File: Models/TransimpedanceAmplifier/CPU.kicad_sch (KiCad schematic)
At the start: 0 parts

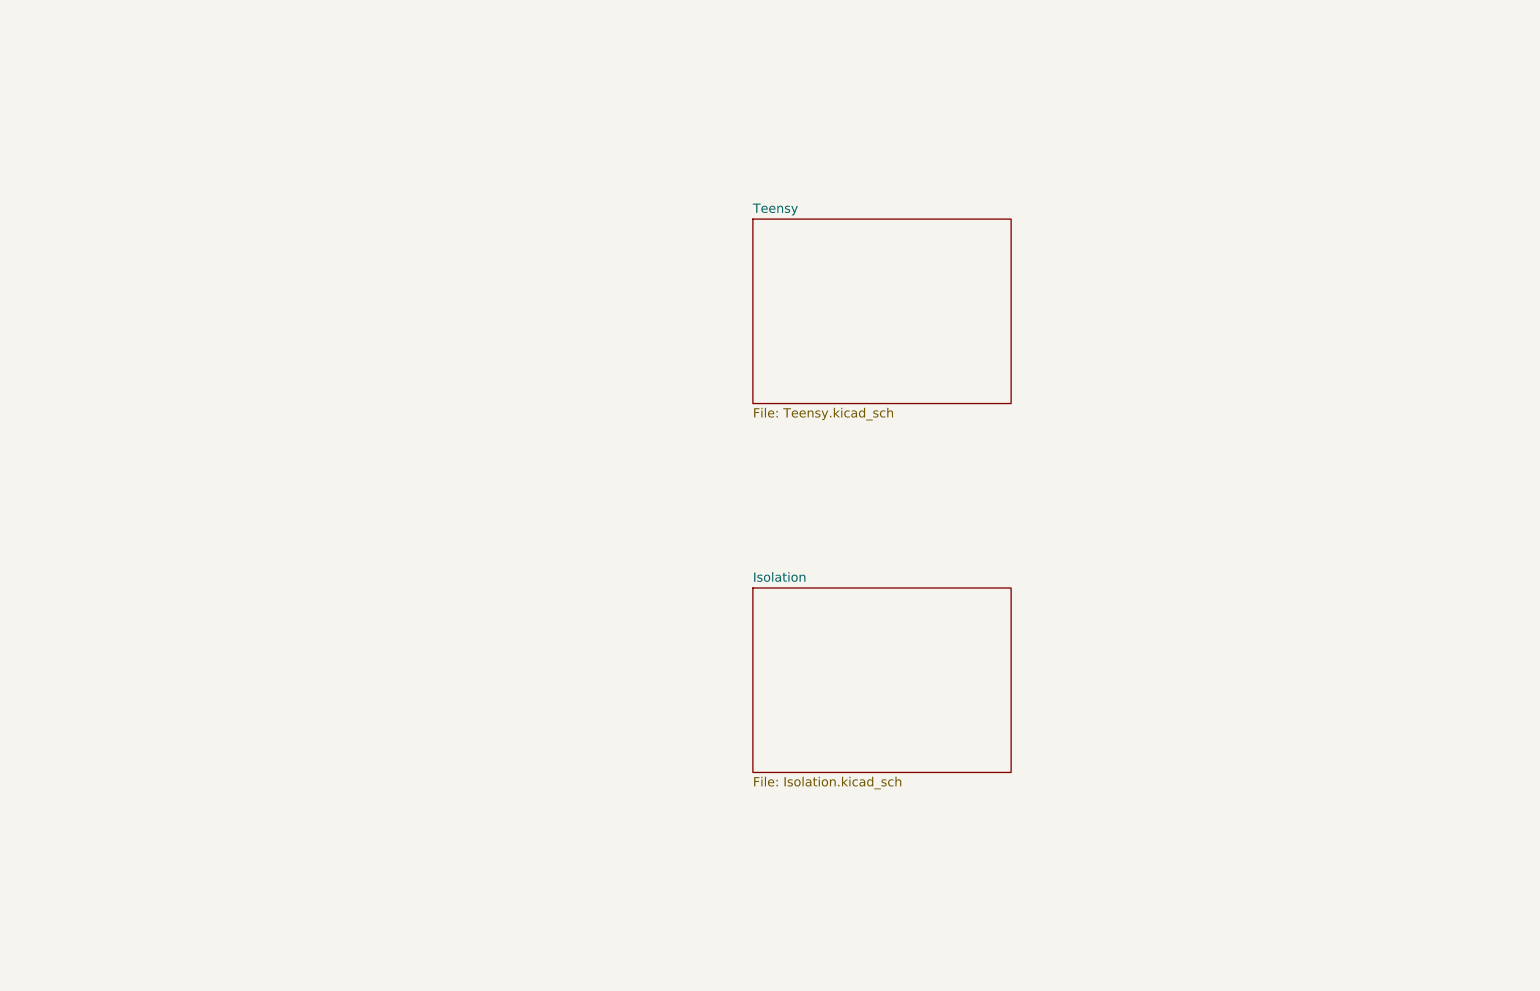
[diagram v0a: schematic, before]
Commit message: Save progress
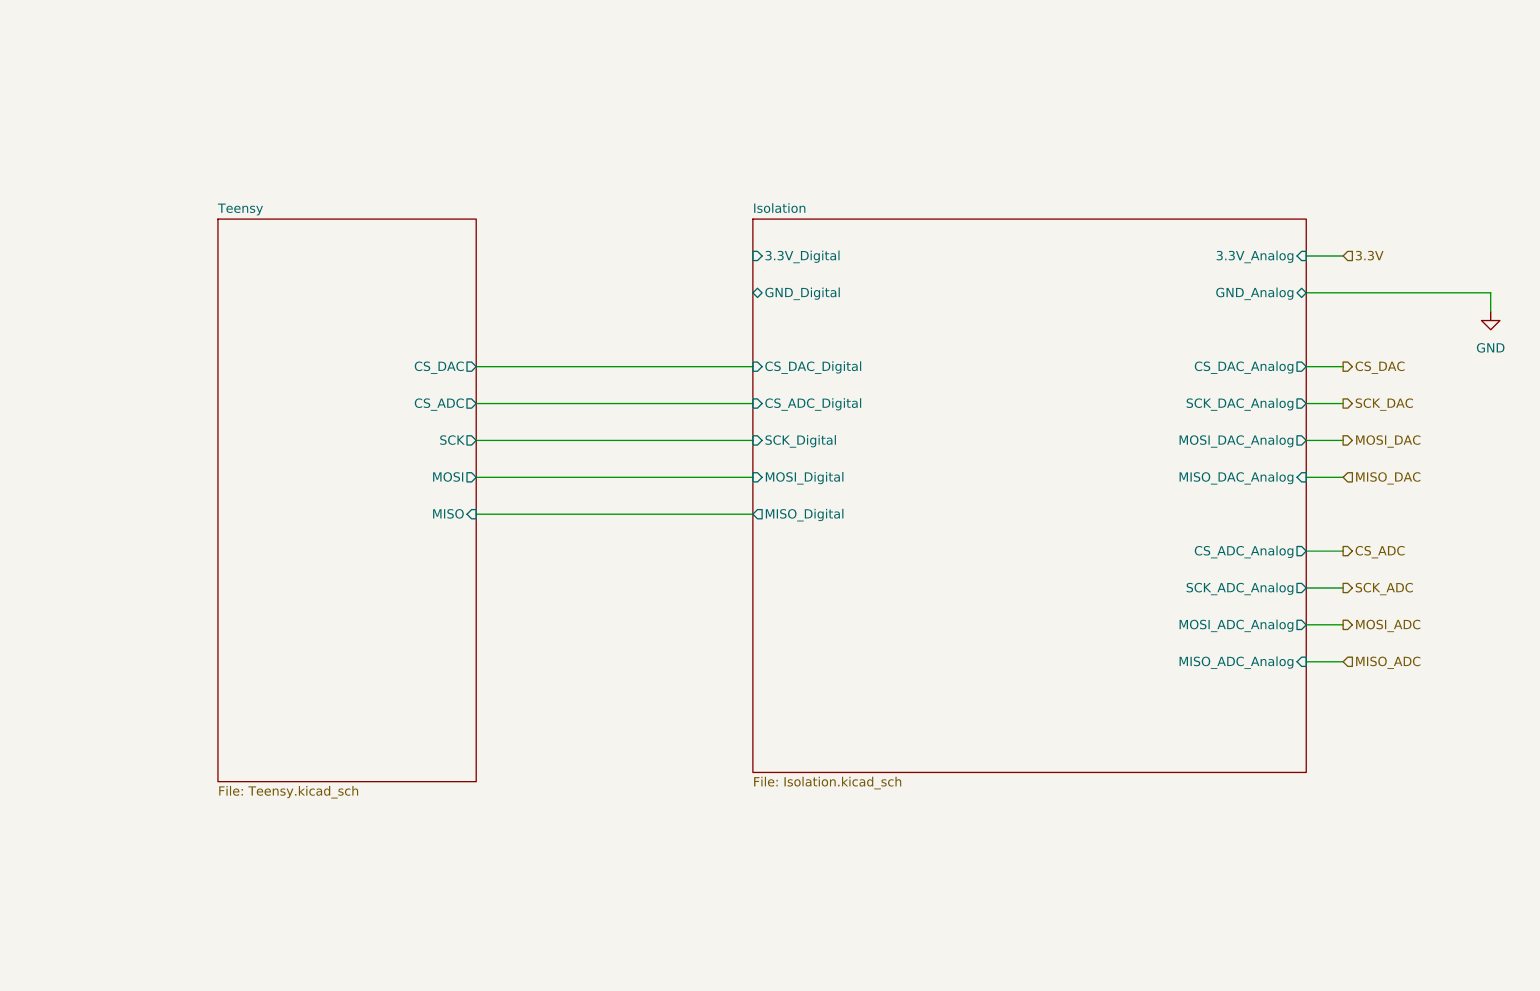
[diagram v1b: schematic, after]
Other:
- sheet Isolation ports: added 3.3V_Analog, 3.3V_Digital, CS_ADC_Analog, CS_ADC_Digital, CS_DAC_Analog, CS_DAC_Digital, GND_Analog, GND_Digital, MISO_ADC_Analog, MISO_DAC_Analog, MISO_Digital, MOSI_ADC_Analog, MOSI_DAC_Analog, MOSI_Digital, SCK_ADC_Analog, SCK_DAC_Analog, SCK_Digital; removed none
- sheet Teensy ports: added CS_ADC, CS_DAC, MISO, MOSI, SCK; removed none

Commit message: Save progress after a major refactoring
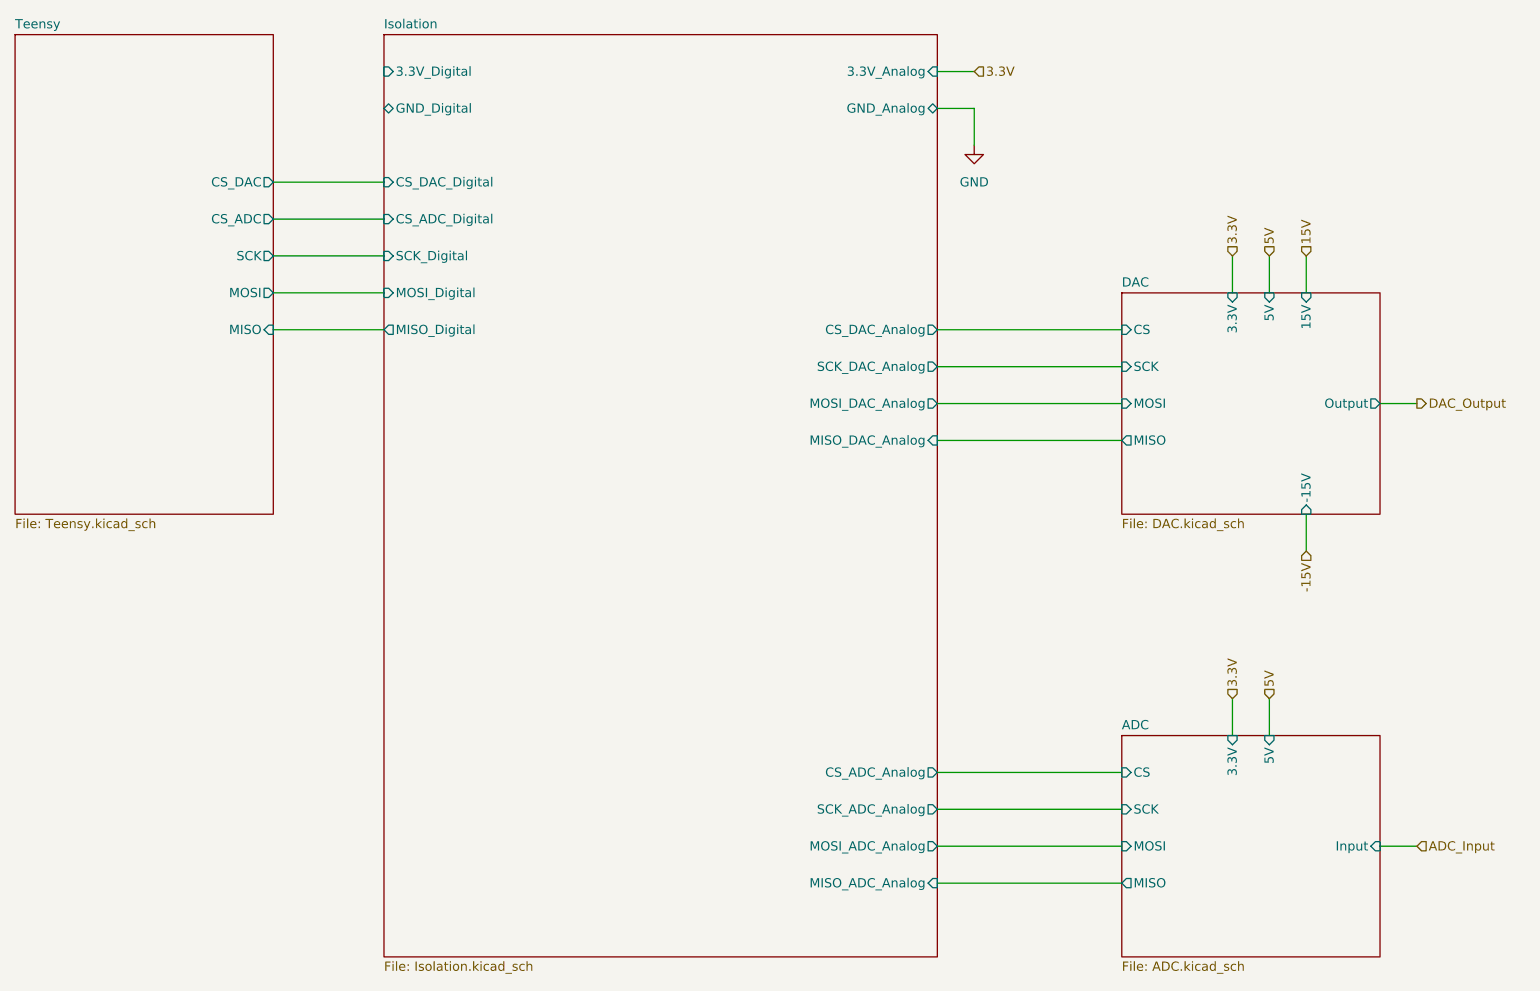
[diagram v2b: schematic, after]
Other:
- added sheet ADC (ADC.kicad_sch)
- added sheet DAC (DAC.kicad_sch)
